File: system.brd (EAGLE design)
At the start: 41.8 x 68.2 mm, 122 parts, among them IC1 TPS7B8650BQDDARQ1, J1 TSW-104-07-F-S, J2 163-179PH-EX, J3 RS1-02-G, SW1 1825910-6, SW2 1825910-6, SW3 1825910-6, U1 ATMEGA328PB-AU, Y1 ABL-16.000MHZ-B2

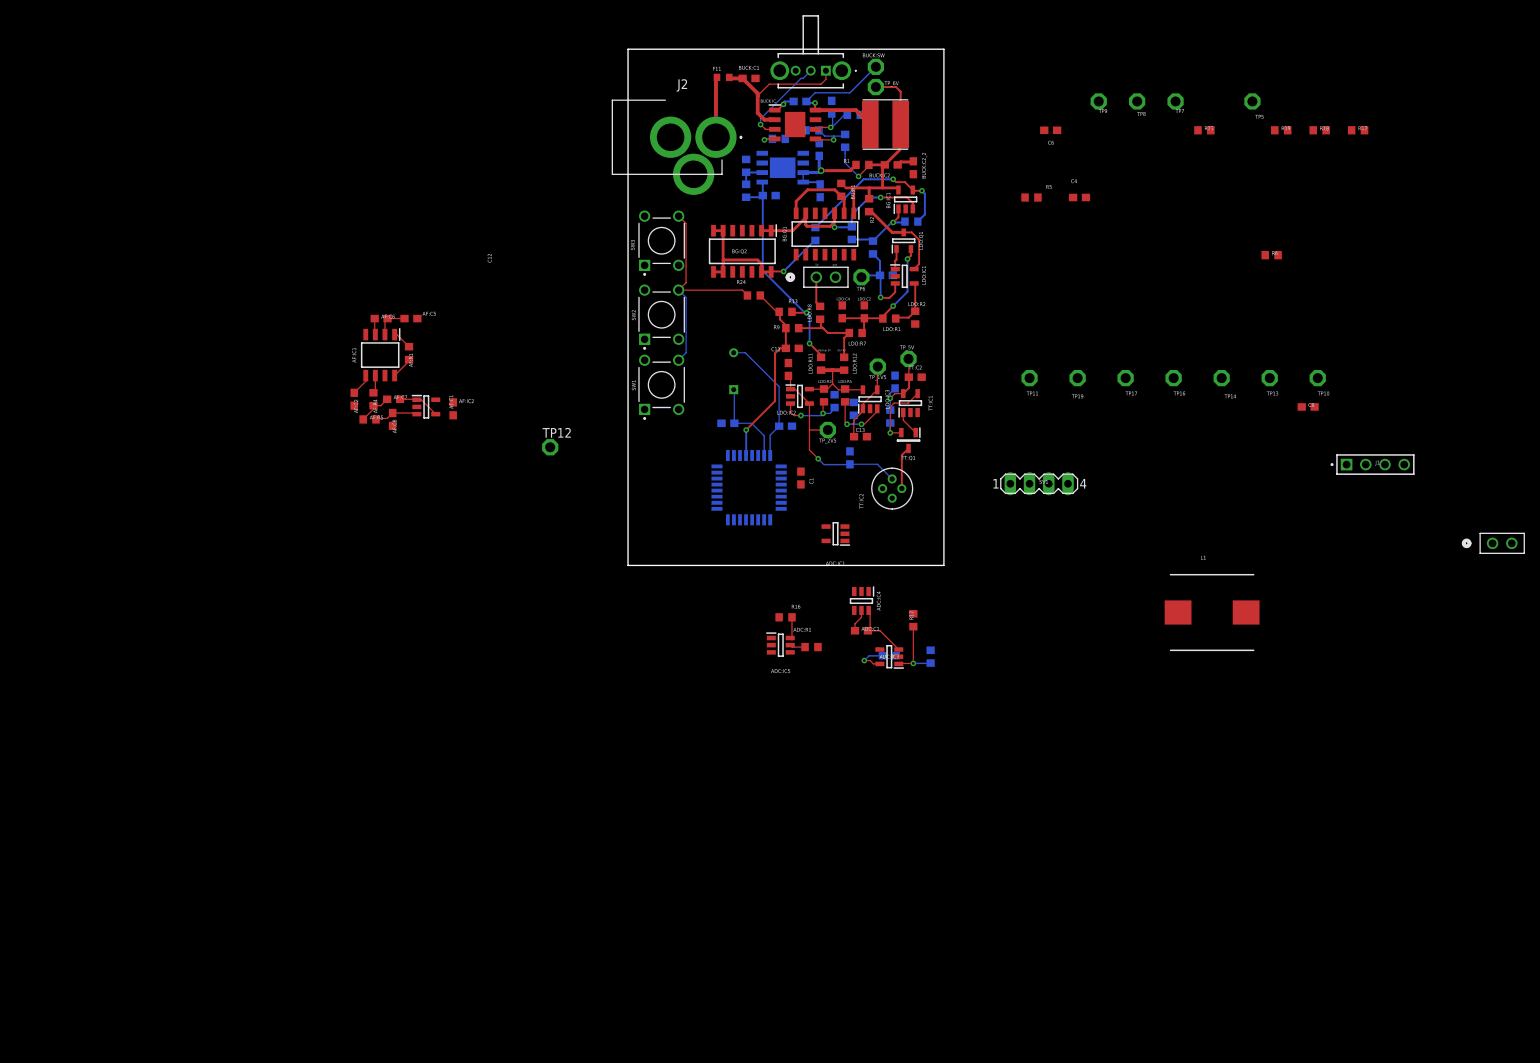
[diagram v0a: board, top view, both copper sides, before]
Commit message: created 3d model for all libraries. routing
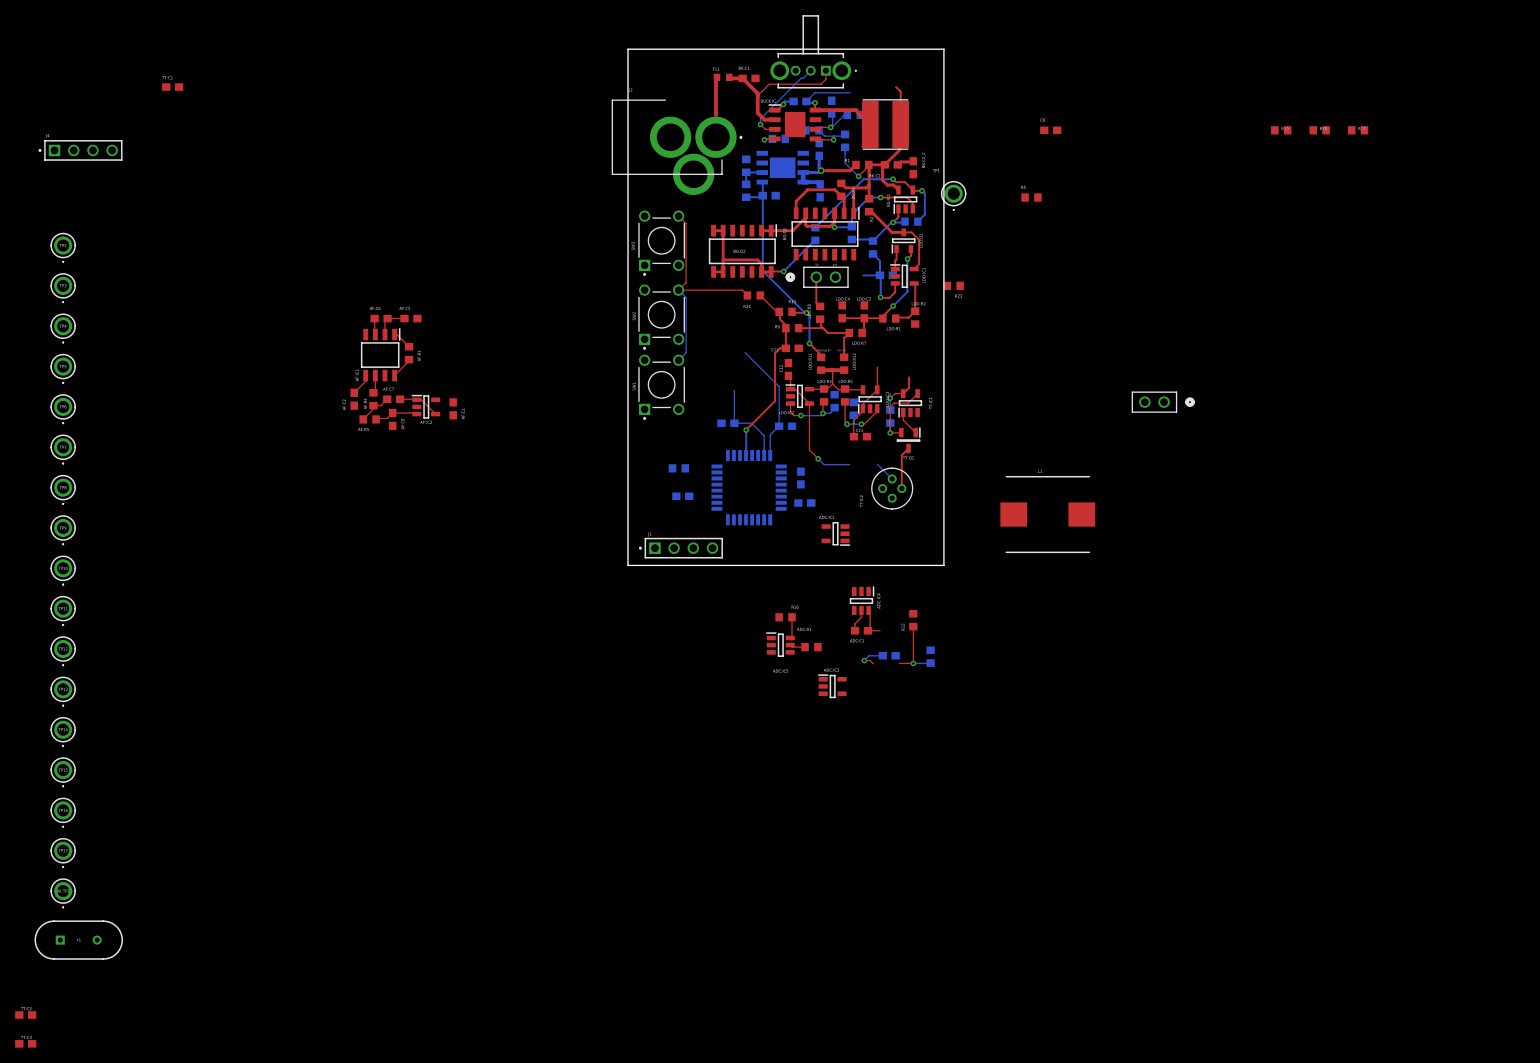
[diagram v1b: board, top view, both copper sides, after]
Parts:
- removed ADC:IC3: TLV9021QDBVRQ1, TLV9021QDBVRQ1:SOT95P280X145-5N
- removed BUCK:SW, TP19, TP_1V5, TP_2V5, TP_5V, TP_6V: TPPAD1-13, testpad:P1-13
- removed SV1: programming pins, con-lstb:MA04-1
- added ADC:IC2: TLV9021QDBVRQ1, TLV9021QDBVRQ1:SOT95P280X145-5N
- added BK:TP1, TP1, TP15, TP2, TP3, TP4: 5010, 5010:5010
- added J4: TSW-104-07-F-S, TSW-104-07-F-S:SAMTEC_TSW-104-07-F-S
- J1: value TSW-104-07-F-S -> OLED
- R5, R6: value 10000 -> 10k
- TP10, TP11, TP12, TP13, TP14, TP16, TP17, TP5, TP6, TP7, TP8, TP9: value TPPAD1-13 -> 5010; device testpad:P1-13 -> 5010:5010
- TT:C1, TT:C2, TT:C3: device BeagleBone_Black_Wireless:C0603 -> resistor:C0603
- moved TP10 167.8 mm to (-75.1, -0.38)
- moved TP13 164.7 mm to (-75.1, -16.4)
- moved TP5 161.1 mm to (-75.1, 26.3)
- moved TP14 160.1 mm to (-75.1, -21.7)
- moved TP16 157.5 mm to (-75.1, -32.4)
- moved TP7 154.0 mm to (-75.1, 15.6)
- moved TP17 153.7 mm to (-75.1, -37.7)
- moved TP8 150.9 mm to (-75.1, 10.3)
- moved TP9 148.1 mm to (-75.1, 4.95)
- moved TT:C2 144.7 mm to (-80.0, -59.4)
- moved TT:C3 133.7 mm to (-80.0, -63.2), flipped to the top, turned to 0 degrees
- moved TP11 131.3 mm to (-75.1, -5.71)
- moved Y1 115.0 mm to (-75.4, -49.5), flipped to the top, turned to 0 degrees
- moved TP6 106.9 mm to (-75.1, 21.0)
- moved TT:C1 103.2 mm to (-60.6, 63.2), flipped to the top, turned to 0 degrees
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- renumbered BUCK:C1 to BK:C1, BUCK:C2 to BK:C2, BUCK:C2_2 to BK:C2_2, BUCK:C3 to BK:C3, BUCK:C5 to BK:C5, BUCK:C6 to BK:C6, BUCK:IC1 to BK:IC1, BUCK:L1 to BK:L1, BUCK:R1 to BK:R1, BUCK:R2 to BK:R2, BUCK:R5 to BK:R5, BUCK:RT to BK:RT, BUCK:S1 to BK:S1
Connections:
- net BUCK:EN renamed BK:EN
- net BUCK:N$1 renamed BK:N$1
- net BUCK:N$3 renamed BK:N$3
- net BUCK:N$4 renamed BK:N$4
- net BUCK:N$5 renamed BK:N$5
- net BUCK:N$6 renamed BK:N$6
- net BUCK:N$7 renamed BK:N$7
- removed net BUCK:N$2: BK:C3.2, BK:IC1.8, BK:L1.1, BUCK:SW.TP
- new net BK:N$2: BK:C3.2, BK:IC1.8, BK:L1.1, BK:TP1.1
- net 0: now also ADC:IC2.2; no longer ADC:IC3.2
- net ADC:N$2: now also ADC:IC2.3; no longer ADC:IC3.3
- net ADC_EXT_INT: now also TP10.1; no longer TP11.TP
- net MCU_RST: now also J4.01, TP15.1; no longer SV1.1, TP17.TP
- net MISO_MCU: now also J4.03, TP12.1; no longer SV1.3, TP13.TP
- net MOSI_MCU: now also J4.02, TP13.1; no longer SV1.2, TP14.TP
- net N$14: now also ADC:IC2.1; no longer ADC:IC3.1
- net N$4: now also TP17.1; no longer TP12.TP
- net N$5: now also ADC:IC2.4; no longer ADC:IC3.4
- net N$6: now also ADC:IC2.5; no longer ADC:IC3.5
- net PB_START: now also TP14.1; no longer TP16.TP
- net RST_ADC: now also TP9.1; no longer TP10.TP
- net SCK_MCU: now also J4.04; no longer SV1.4
- net SDA: now also TP16.1; no longer TP19.TP
- net VS_1.5V_OUT: now also TP4.1; no longer TP_1V5.TP
- net VS_2.5V_OUT: now also TP3.1; no longer TP_2V5.TP
- net VS_5V_OUT: now also TP2.1; no longer TP_5V.TP
- net VS_6V: now also TP1.1; no longer TP_6V.TP
- net V_BG: now also TP6.1; no longer TP6.TP
- net V_SIG: now also TP8.1; no longer TP9.TP
- net V_TH: now also TP5.1; no longer TP5.TP
- net V_TOGGLE: now also TP11.1; no longer TP8.TP
- net V_TP: now also TP7.1; no longer TP7.TP
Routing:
- net BUCK:N$2: track 21.3 -> 0.00 mm, vias 1 -> 0
- net BK:N$2: track 0.00 -> 16.5 mm, vias 0 -> 1
- net VS_2.5V_OUT: track 33.7 -> 27.6 mm
- net ADC:N$2: track 7.88 -> 4.37 mm
- net VS_5V_OUT: track 35.6 -> 32.3 mm
- net VS_6V: track 38.6 -> 36.9 mm
- net EXT_CLK_2: track 17.5 -> 15.9 mm
- net N$6: track 4.95 -> 4.10 mm

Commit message: routing
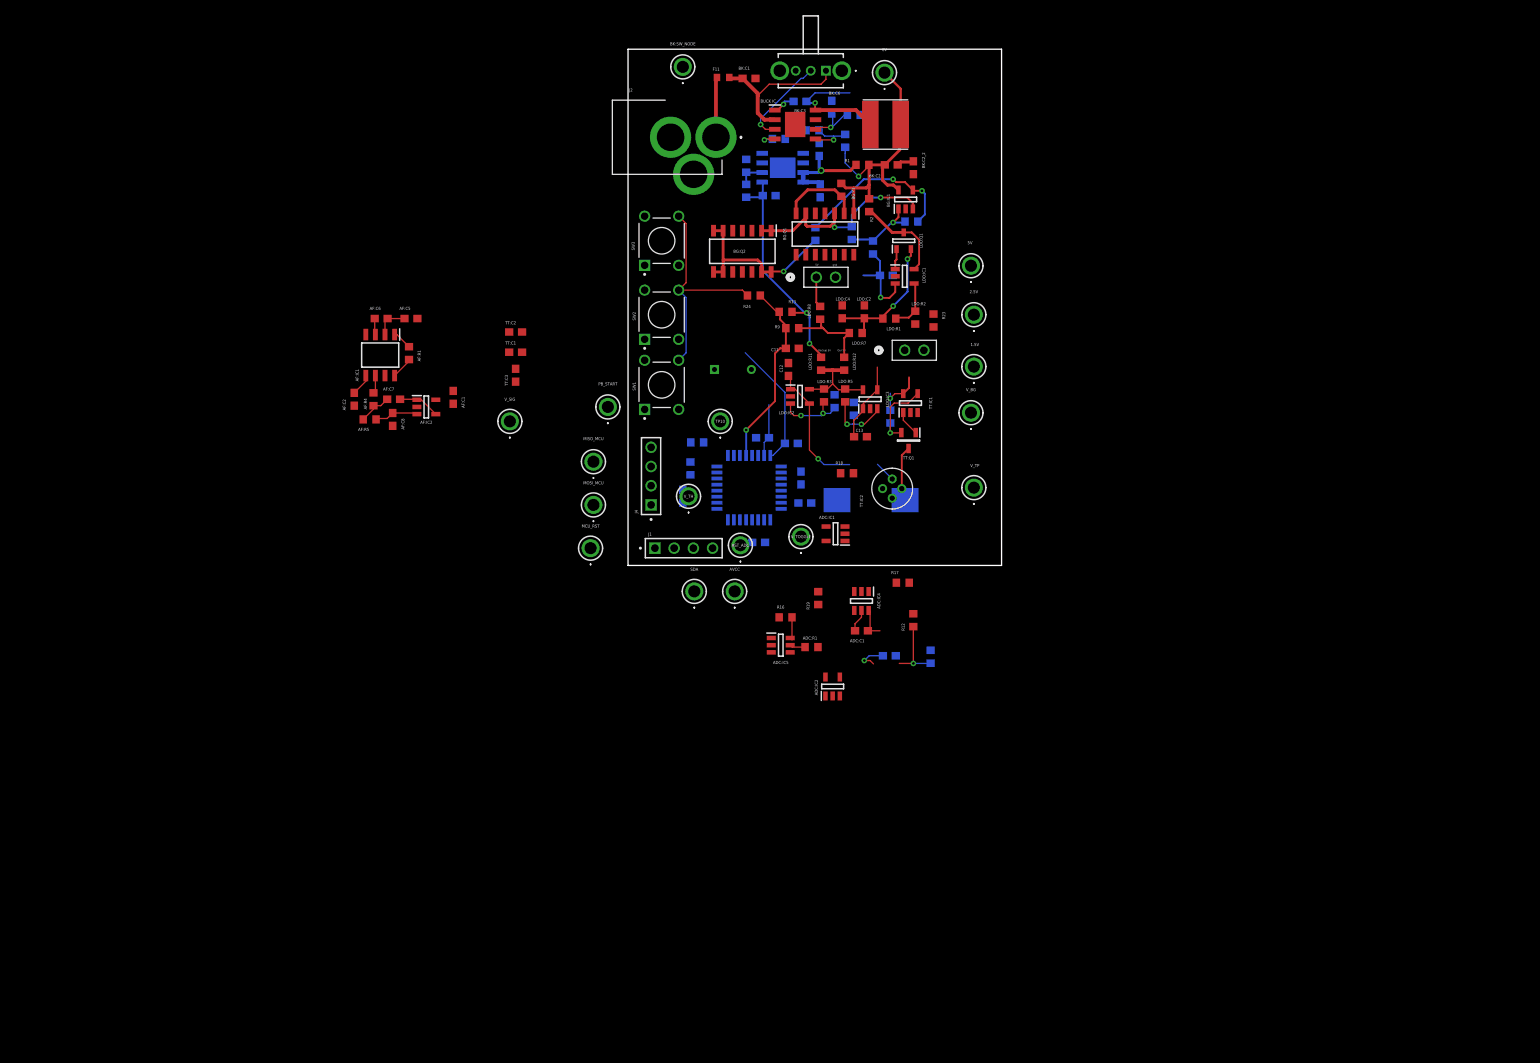
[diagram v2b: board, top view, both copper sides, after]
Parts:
- removed BK:TP1, TP1, TP11, TP12, TP13, TP14, TP15, TP16, TP17, TP2, TP3, TP4, TP5, TP6, TP7, TP8, TP9: 5010, 5010:5010
- added 1.5V, 2.5V, 5V, 6V, AVCC, BK:SW_NODE, MCU_RST, MISO_MCU, MOSI_MCU, PB_START, RST_ADC, SDA, V_BG, V_SIG, V_TH, V_TOGGLE, V_TP: 5010, 5010:5010
- J3: value RS1-02-G -> AD2
- J4: value TSW-104-07-F-S -> MCU
- moved Y1 114.8 mm to (11.0, 25.9), flipped to the bottom, turned to 180 degrees
- moved TT:C2 111.1 mm to (-15.2, 30.9)
- moved TT:C3 109.6 mm to (-15.2, 25.1), turned to 90 degrees
- moved TP10 89.0 mm to (11.8, 19.1)
- moved R19 87.0 mm to (24.8, -4.32), turned to 90 degrees
- moved J4 86.5 mm to (2.67, 11.8), turned to 90 degrees
- moved R17 84.9 mm to (35.9, -2.29)
- moved R18 77.2 mm to (28.6, 12.2)
- moved C6 66.8 mm to (16.9, 3.05), flipped to the bottom
- moved TT:C1 57.3 mm to (-15.2, 28.2)
- moved R5 54.8 mm to (8.76, 16.3), flipped to the bottom
- moved J3 35.0 mm to (36.2, 28.4), turned to 0 degrees
- moved L1 23.4 mm to (31.8, 8.64), flipped to the bottom
- moved R23 5.29 mm to (40.0, 32.4), turned to 270 degrees
- moved C9 4.95 mm to (17.4, 16.9)
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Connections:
- net BK:N$2: now also BK:SW_NODE.1; no longer BK:TP1.1
- net MCU_RST: now also MCU_RST.1; no longer TP15.1
- net MISO_MCU: now also MISO_MCU.1; no longer TP12.1
- net MOSI_MCU: now also MOSI_MCU.1; no longer TP13.1
- net N$4: now also AVCC.1; no longer TP17.1
- net PB_START: now also PB_START.1; no longer TP14.1
- net RST_ADC: now also RST_ADC.1; no longer TP9.1
- net SDA: now also SDA.1; no longer TP16.1
- net VS_1.5V_OUT: now also 1.5V.1; no longer TP4.1
- net VS_2.5V_OUT: now also 2.5V.1; no longer TP3.1
- net VS_5V_OUT: now also 5V.1; no longer TP2.1
- net VS_6V: now also 6V.1; no longer TP1.1
- net V_BG: now also V_BG.1; no longer TP6.1
- net V_SIG: now also V_SIG.1; no longer TP8.1
- net V_TH: now also V_TH.1; no longer TP5.1
- net V_TOGGLE: now also V_TOGGLE.1; no longer TP11.1
- net V_TP: now also V_TP.1; no longer TP7.1
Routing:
- net EXT_CLK_1: track 11.7 -> 7.06 mm
- net VS_6V: track 36.9 -> 39.4 mm
- net EXT_CLK_2: track 15.9 -> 16.8 mm
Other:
- board size 41.8 x 68.2 mm -> 49.4 x 68.2 mm
